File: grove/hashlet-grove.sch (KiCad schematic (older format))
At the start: 2 parts, among them P1 TWIG_2.0, U1 ATSHA204A

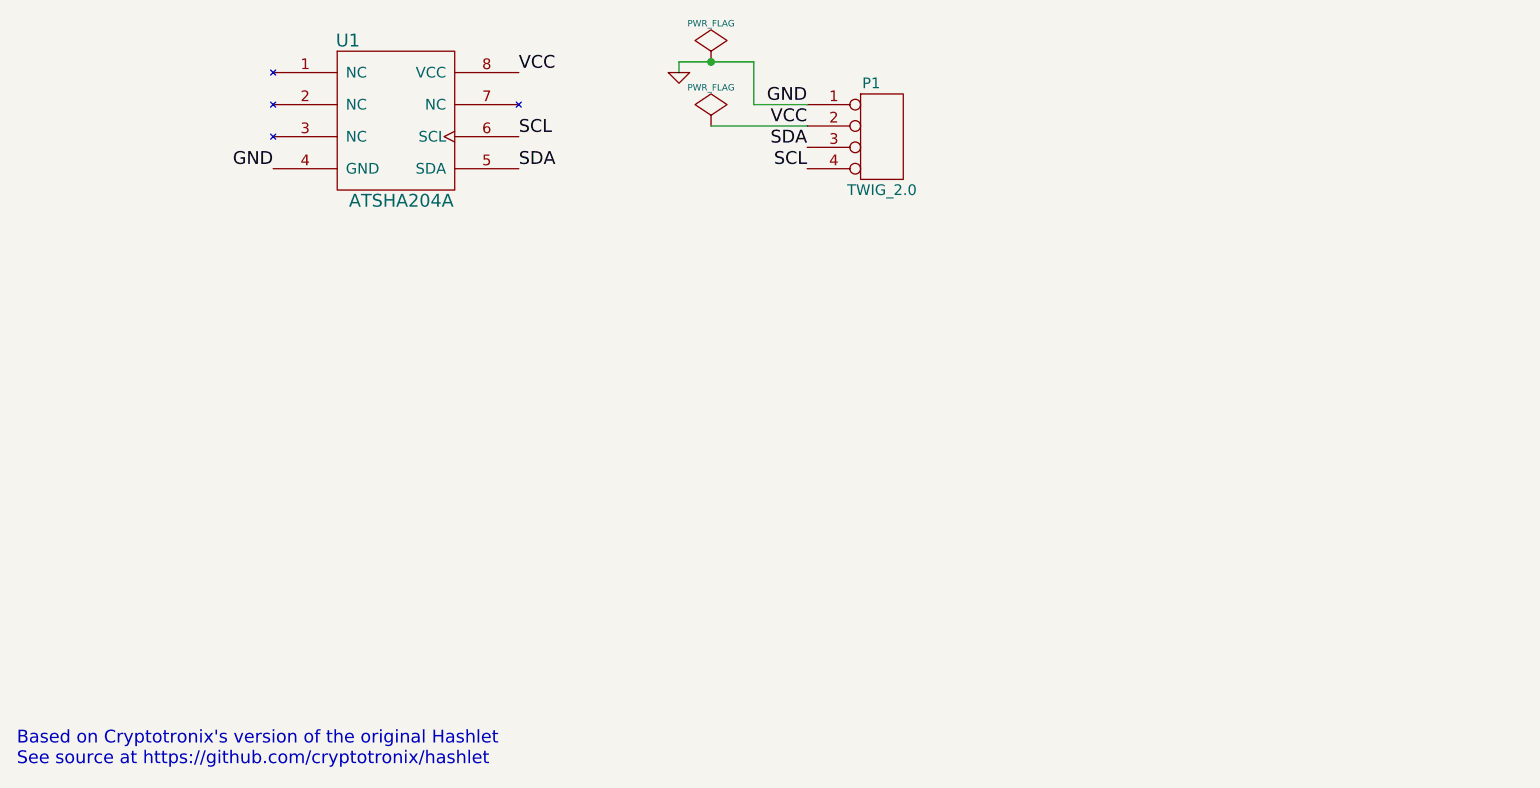
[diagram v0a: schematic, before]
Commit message: Hashlet for Grove rev v1
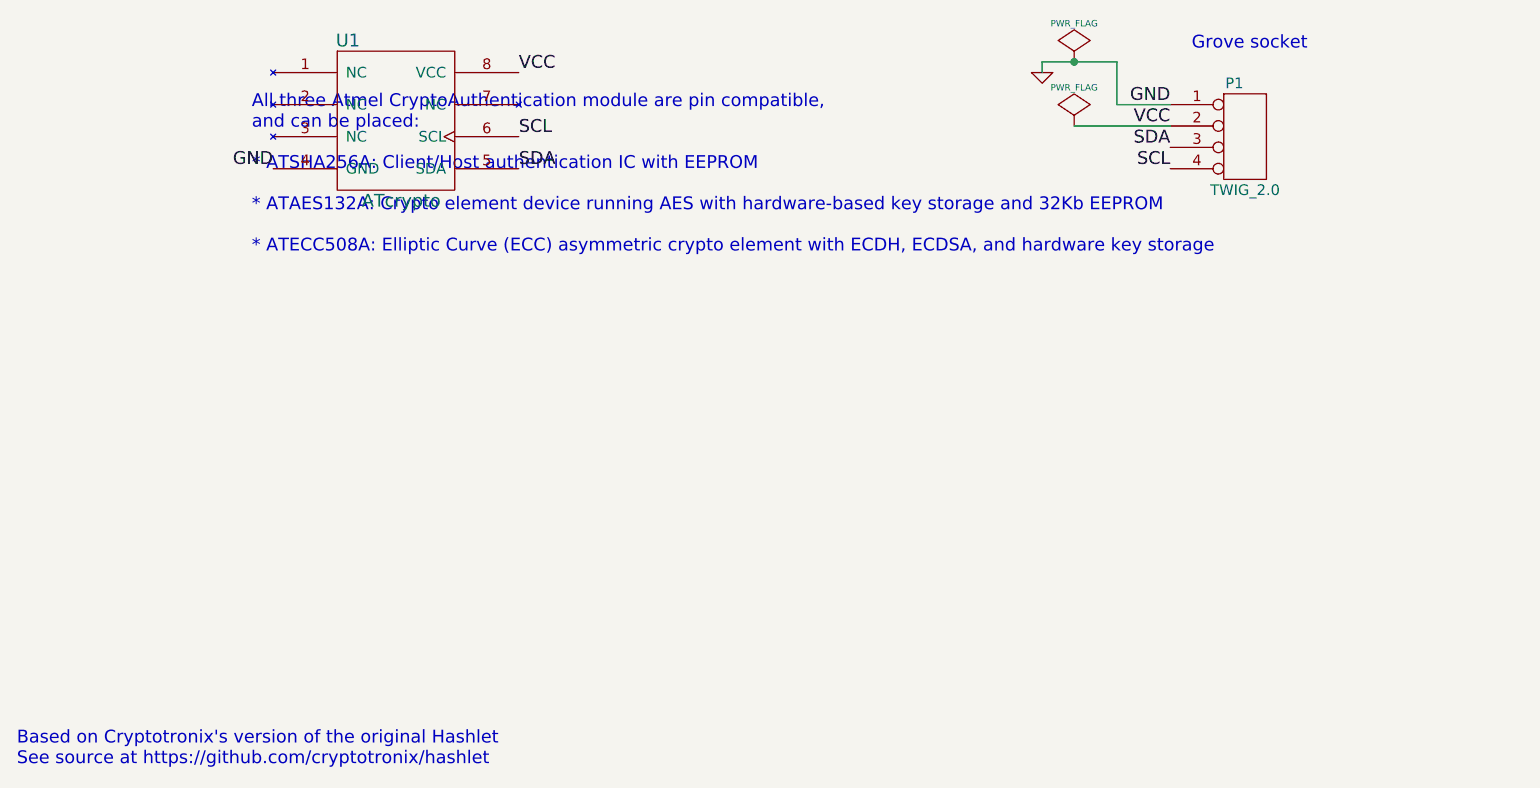
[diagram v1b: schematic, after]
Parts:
- P1: S1N (none) -> Seeed
- U1: value ATSHA204A -> ATcrypto; MFP ATSHA204A-SSHDA-T -> (none); MFPN (none) -> ATSHA204A / ATAES132A / ATECC508A; S1PL https://www.mouser.tw/Search/ProductDetail.aspx?R=ATSHA204A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 -> (none); S1PN 556-ATSHA204A-SSHDAT -> (none); S2PL http://www.digikey.com/product-detail/en/ATSHA204A-SSHDA-T/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 -> (none); S2PN ATSHA204A-SSHDA-TCT-ND -> (none)
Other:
- note added: "All three Atmel CryptoAuthentication module are pin compatible,\nand can be placed:\n\n* ATSHA256A: Client/Host authentication IC with EEPROM\n\n* ATAES132A: Crypto element device running AES with hardware-based key storage and 32Kb EEPROM\n\n* ATECC508A: Elliptic Curve (ECC) asymmetric crypto element with ECDH, ECDSA, and hardware key storage"
- note added: "Grove socket"
- moved on the sheet: P1
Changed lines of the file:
@@
 Sheet 1 1
 Title "Hashlet for Grove"
-Date "9 aug 2015"
+Date "15 aug 2015"
 Rev "1"
 Comp "Gergely Imreh / Moonpunch"
@@
 P 4800 3900
 F 0 "U1" H 4500 4250 60  0000 C CNN
-F 1 "ATSHA204A" H 4750 3500 60  0000 C CNN
+F 1 "ATcrypto" H 4750 3500 60  0000 C CNN
 F 2 "so-8" H 4800 3900 60  0001 C CNN
-F 3 "http://www.atmel.com/Images/Atmel-8885-CryptoAuth-ATSHA204A-Datasheet.pdf" H 4800 3900 60  0001 C CNN
+F 3 "http://www.atmel.com/products/security-ics/cryptoauthentication/default.aspx" H 4800 3900 60  0001 C CNN
 F 4 "Atmel" H 4800 3900 60  0001 C CNN "MFN"
-F 5 "ATSHA204A-SSHDA-T" H 4800 3900 60  0001 C CNN "MFP"
-F 6 "556-ATSHA204A-SSHDAT" H 4800 3900 60  0001 C CNN "S1PN"
-F 7 "https://www.mouser.tw/Search/ProductDetail.aspx?R=ATSHA204A-SSHDA-Tvirtualkey55660000virtualkey556-ATSHA204A-SSHDAT" H 4800 3900 60  0001 C CNN "S1PL"
-F 8 "ATSHA204A-SSHDA-TCT-ND" H 4800 3900 60  0001 C CNN "S2PN"
-F 9 "http://www.digikey.com/product-detail/en/ATSHA204A-SSHDA-T/ATSHA204A-SSHDA-TCT-ND/4814556" H 4800 3900 60  0001 C CNN "S2PL"
+F 5 "ATSHA204A / ATAES132A / ATECC508A" H 4800 3900 60  0001 C CNN "MFPN"
 	1    4800 3900
 	1    0    0    -1
@@
 Text Label 4150 4150 2    60   ~ 0
 GND
-Text Label 6650 3850 2    60   ~ 0
+Text Label 8350 3850 2    60   ~ 0
 GND
-Text Label 6650 4050 2    60   ~ 0
+Text Label 8350 4050 2    60   ~ 0
 SDA
-Text Label 6650 4150 2    60   ~ 0
+Text Label 8350 4150 2    60   ~ 0
 SCL
 $Comp
 L PWR_FLAG #FLG01
 U 1 1 546861FB
-P 6200 3950
-F 0 "#FLG01" H 6200 4045 30  0001 C CNN
-F 1 "PWR_FLAG" H 6200 4130 30  0000 C CNN
-F 2 "" H 6200 3950 60  0000 C CNN
-F 3 "" H 6200 3950 60  0000 C CNN
-	1    6200 3950
+P 7900 3950
+F 0 "#FLG01" H 7900 4045 30  0001 C CNN
+F 1 "PWR_FLAG" H 7900 4130 30  0000 C CNN
+F 2 "" H 7900 3950 60  0000 C CNN
+F 3 "" H 7900 3950 60  0000 C CNN
+	1    7900 3950
 	1    0    0    -1
 $EndComp
@@
 L GND #PWR02
 U 1 1 5468620A
-P 6050 3700
-F 0 "#PWR02" H 6050 3700 30  0001 C CNN
-F 1 "GND" H 6050 3630 30  0001 C CNN
-F 2 "" H 6050 3700 60  0000 C CNN
-F 3 "" H 6050 3700 60  0000 C CNN
-	1    6050 3700
+P 7750 3700
+F 0 "#PWR02" H 7750 3700 30  0001 C CNN
+F 1 "GND" H 7750 3630 30  0001 C CNN
+F 2 "" H 7750 3700 60  0000 C CNN
+F 3 "" H 7750 3700 60  0000 C CNN
+	1    7750 3700
 	1    0    0    -1
 $EndComp
@@
 L PWR_FLAG #FLG03
 U 1 1 54686219
-P 6200 3650
-F 0 "#FLG03" H 6200 3745 30  0001 C CNN
-F 1 "PWR_FLAG" H 6200 3830 30  0000 C CNN
-F 2 "" H 6200 3650 60  0000 C CNN
-F 3 "" H 6200 3650 60  0000 C CNN
-	1    6200 3650
+P 7900 3650
+F 0 "#FLG03" H 7900 3745 30  0001 C CNN
+F 1 "PWR_FLAG" H 7900 3830 30  0000 C CNN
+F 2 "" H 7900 3650 60  0000 C CNN
+F 3 "" H 7900 3650 60  0000 C CNN
+	1    7900 3650
 	1    0    0    -1
 $EndComp
 Wire Wire Line
-	6050 3700 6050 3650
+	7750 3700 7750 3650
 Wire Wire Line
-	6050 3650 6400 3650
+	7750 3650 8100 3650
 Text Notes 2950 6950 0    60   ~ 0
 Based on Cryptotronix's version of the original Hashlet\nSee source at https://github.com/cryptotronix/hashlet
-Text Label 6650 3950 2    60   ~ 0
+Text Label 8350 3950 2    60   ~ 0
 VCC
 $Comp
 L CONN_4 P1
 U 1 1 55C6ED69
-P 7000 4000
-F 0 "P1" H 6950 4250 50  0000 C CNN
-F 1 "TWIG_2.0" H 7000 3750 50  0000 C CNN
-F 2 "TWIG_2.0" H 7000 4000 60  0001 C CNN
-F 3 "http://www.seeedstudio.com/depot/images/opl/datasheet/3470130P1.pdf" H 7000 4000 60  0001 C CNN
-F 4 "Taifeng" H 7000 4000 60  0001 C CNN "MFN"
-F 5 "1125S-4P" H 7000 4000 60  0001 C CNN "MFPN"
-F 6 "320110033" H 7000 4000 60  0001 C CNN "S1PN"
-F 7 "http://www.seeedstudio.com/depot/index.php?main_page=opl_info&opl_id=4" H 7000 4000 60  0001 C CNN "S1L"
-	1    7000 4000
+P 8700 4000
+F 0 "P1" H 8650 4250 50  0000 C CNN
+F 1 "TWIG_2.0" H 8700 3750 50  0000 C CNN
+F 2 "TWIG_2.0" H 8700 4000 60  0001 C CNN
+F 3 "http://www.seeedstudio.com/depot/images/opl/datasheet/3470130P1.pdf" H 8700 4000 60  0001 C CNN
+F 4 "Taifeng" H 8700 4000 60  0001 C CNN "MFN"
+F 5 "1125S-4P" H 8700 4000 60  0001 C CNN "MFPN"
+F 6 "Seeed" H 8700 4000 60  0001 C CNN "S1N"
+F 7 "320110033" H 8700 4000 60  0001 C CNN "S1PN"
+F 8 "http://www.seeedstudio.com/depot/index.php?main_page=opl_info&opl_id=4" H 8700 4000 60  0001 C CNN "S1L"
+	1    8700 4000
 	1    0    0    -1
 $EndComp
 Wire Wire Line
-	6650 3950 6200 3950
+	8350 3950 7900 3950
 Wire Wire Line
-	6400 3650 6400 3850
+	8100 3650 8100 3850
 Wire Wire Line
-	6400 3850 6650 3850
-Connection ~ 6200 3650
+	8100 3850 8350 3850
+Connection ~ 7900 3650
+Text Notes 4050 4550 0    60   ~ 0
+All three Atmel CryptoAuthentication module are pin compatible,\nand can be placed:\n\n* ATSHA256A: Client/Host authentication IC with EEPROM\n\n* ATAES132A: Crypto element device running AES with hardware-based key storage and 32Kb EEPROM\n\n* ATECC508A: Elliptic Curve (ECC) asymmetric crypto element with ECDH, ECDSA, and hardware key storage
+Text Notes 8450 3600 0    60   ~ 0
+Grove socket
 $EndSCHEMATC
